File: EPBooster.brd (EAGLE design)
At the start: 51.1 x 27.3 mm, 33 parts, among them Q1 2N5457, Q2 2N5088, SW1 DIP 2 POS

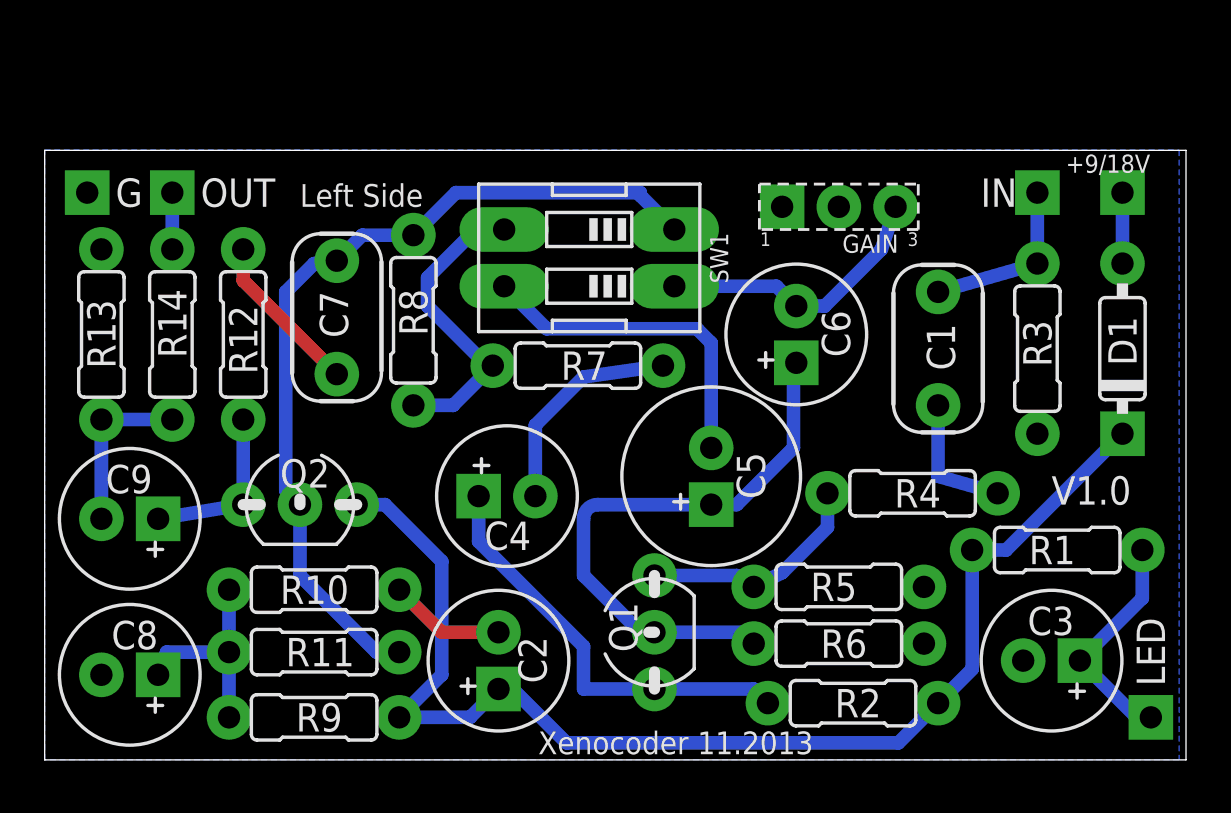
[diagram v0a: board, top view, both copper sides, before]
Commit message: New Board and Schematic for v1.2
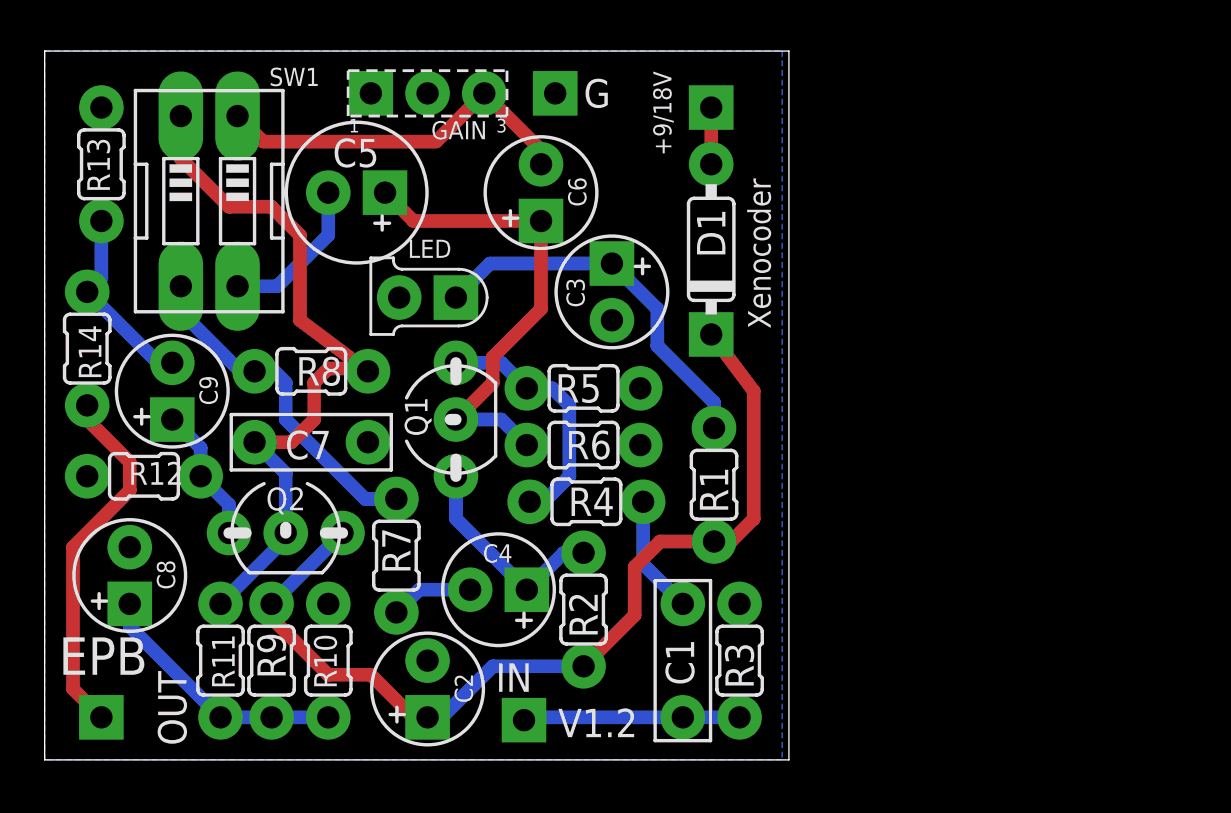
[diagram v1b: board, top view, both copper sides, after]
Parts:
- C1, C7: device mb_caps-chicklet:075X040 -> mb_caps-box:072X025
- C2, C3, C4, C6, C8, C9: device mb_caps-electro:063_025 -> mb_caps-electro:050_020_1
- C5: device mb_caps-electro:080_035_1 -> mb_caps-electro:063_025
- LED: value 3mm -> 3MM; device mb_supply:SQUARE -> mb_diodes:LED3MM
- R1, R10, R11, R12, R13, R14, R2, R3, R4, R5, R6, R7, R8, R9: device mb_resistors:R0207/3 -> mb_resistors:R0204/2
- moved LED 37.4 mm to (17.1, 20.7), turned to 180 degrees
- moved IN 33.0 mm to (21.5, 1.78)
- moved C3 25.7 mm to (25.4, 21.0), turned to 270 degrees
- moved OUT 23.7 mm to (2.54, 1.91)
- moved G 21.4 mm to (22.9, 29.8)
- moved C5 20.3 mm to (14.0, 25.4), turned to 180 degrees
- moved R3 19.3 mm to (31.1, 4.45), turned to 90 degrees
- moved GAIN 19.1 mm to (17.1, 29.8)
- moved D1 18.9 mm to (29.8, 22.9)
- moved +9/18V 18.8 mm to (29.8, 29.2)
- moved C1 18.1 mm to (28.6, 4.45), turned to 90 degrees
- moved SW1 17.2 mm to (7.37, 25.0), turned to 180 degrees
- moved R1 15.6 mm to (30.0, 12.3), turned to 90 degrees
- moved R4 14.6 mm to (24.3, 11.6)
- moved R5 14.5 mm to (24.1, 16.6)
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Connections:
- net GND: now also LED.K
- net N$1: now also LED.A; no longer LED.1
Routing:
- net OUT: track 2.54 -> 16.3 mm
- net N$2: track 55.4 -> 42.4 mm
- net GND: track 12.6 -> 0.00 mm
- net N$5: track 19.1 -> 9.62 mm
- net N$8: track 15.0 -> 6.92 mm
- net N$1: track 10.3 -> 16.9 mm
- net N$7: track 9.82 -> 3.72 mm
- net N$15: track 38.8 -> 32.8 mm
- net N$6: track 26.0 -> 21.6 mm
- net N$10: track 12.7 -> 16.6 mm
- net IN: track 7.80 -> 9.70 mm
- net N$9: track 7.67 -> 6.13 mm
- net N$11: track 13.9 -> 15.3 mm
- net N$13: track 10.5 -> 11.6 mm
- net N$4: track 10.4 -> 11.4 mm
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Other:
- board size 51.1 x 27.3 mm -> 33.3 x 31.7 mm
- board text added: "EPB"
- board text added: "V1.2"
- board text added: "Xenocoder"
- board text removed: "Left Side"
- board text removed: "V1.0"
- board text removed: "Xenocoder 11.2013"
